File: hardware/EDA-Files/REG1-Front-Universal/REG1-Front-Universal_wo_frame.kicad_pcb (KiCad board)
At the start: 2 copper layers, 15.3 x 42.6 mm, 18 parts, among them J1 Frontpanel, SW1 Prog, SW2 Btn1, SW3 Res, SW4 BL

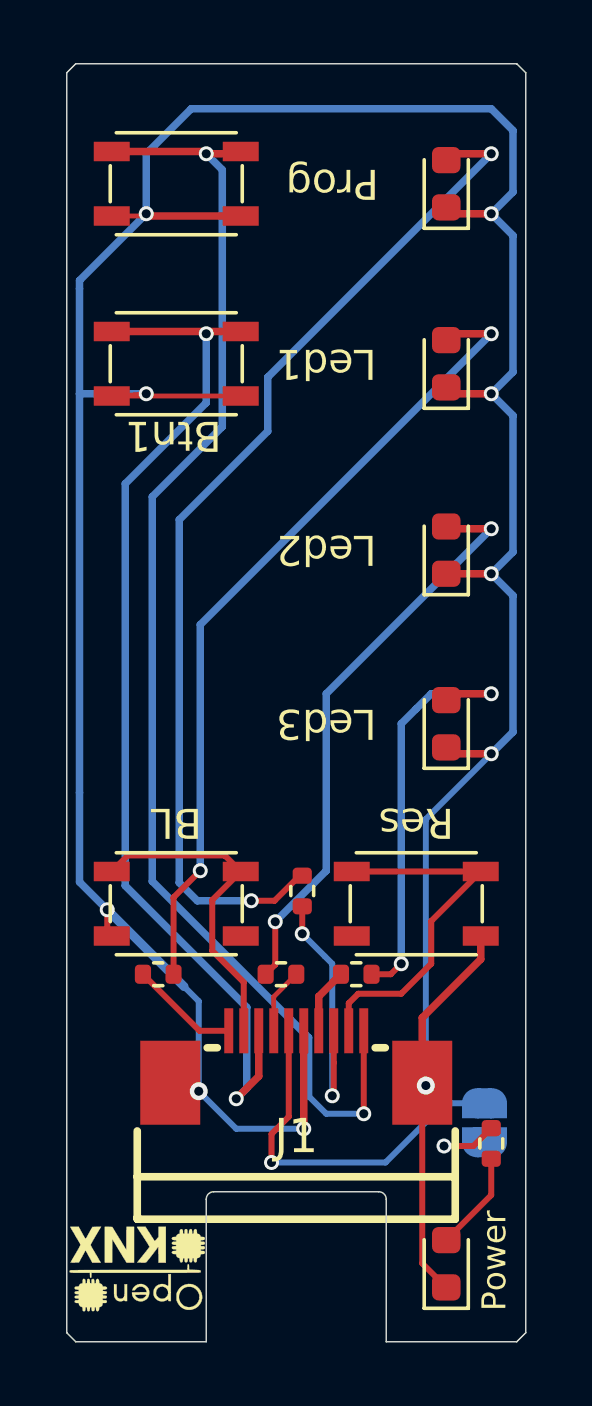
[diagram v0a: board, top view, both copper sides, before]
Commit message: new V01.00 (some 0.1 bigger)
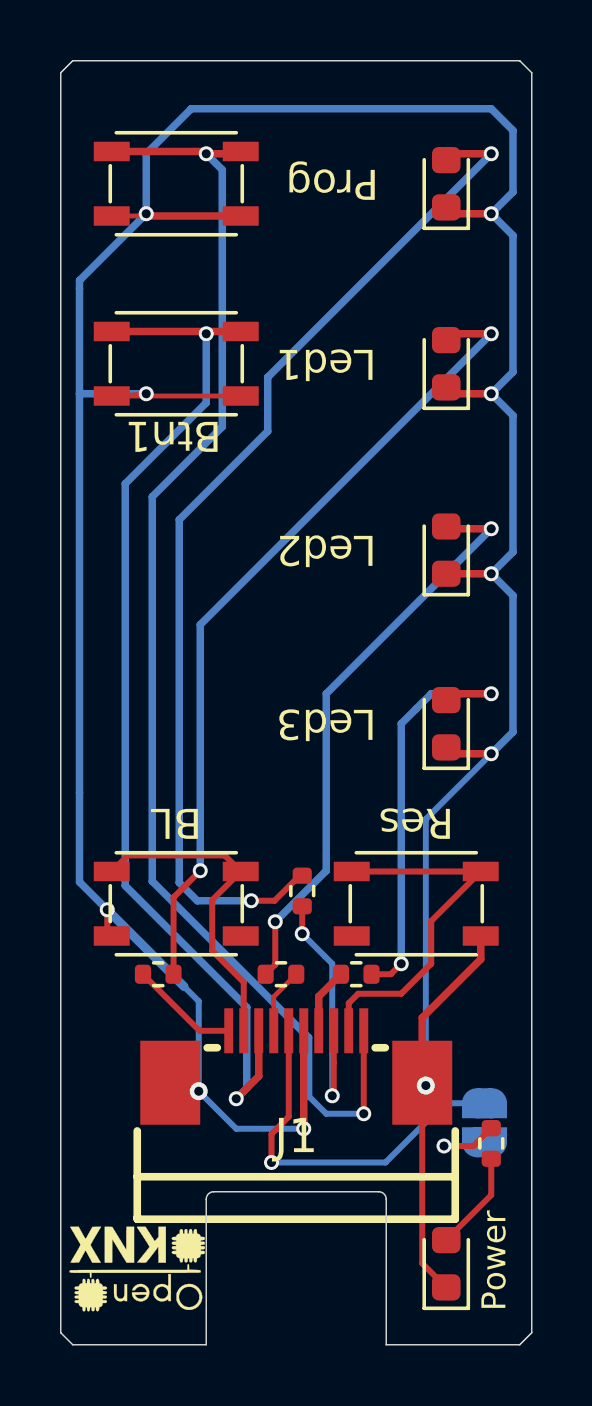
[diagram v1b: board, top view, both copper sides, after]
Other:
- board size 15.3 x 42.6 mm -> 15.7 x 42.8 mm
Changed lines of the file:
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@@
       (drillshape 0)
       (scaleselection 1)
-      (outputdirectory "REG1-Front-Universal_gerbers_V01.00/")
+      (outputdirectory "dxf/")
     )
   )
@@
   (gr_line (start 58.325 83) (end 60.225 83)
     (stroke (width 0.1) (type default)) (layer "Eco1.User"))
-  (gr_line (start 46.35 85.3) (end 46.35 43.3)
+  (gr_line (start 46.15 85.3) (end 46.15 43.3)
     (stroke (width 0.05) (type solid)) (layer "Edge.Cuts"))
-  (gr_line (start 61.35 43) (end 46.65 43)
+  (gr_line (start 61.45 85.7) (end 57 85.7)
+    (stroke (width 0.05) (type solid)) (layer "Edge.Cuts"))
+  (gr_line (start 51 85.7) (end 46.55 85.7)
+    (stroke (width 0.05) (type solid)) (layer "Edge.Cuts"))
+  (gr_line (start 61.45 42.9) (end 46.55 42.9)
     (stroke (width 0.05) (type default)) (layer "Edge.Cuts"))
-  (gr_line (start 46.65 43) (end 46.35 43.3)
+  (gr_line (start 46.55 42.9) (end 46.15 43.3)
     (stroke (width 0.05) (type solid)) (layer "Edge.Cuts"))
-  (gr_line (start 61.65 85.3) (end 61.35 85.6)
+  (gr_line (start 61.85 85.3) (end 61.45 85.7)
     (stroke (width 0.05) (type solid)) (layer "Edge.Cuts"))
-  (gr_line (start 46.65 85.6) (end 46.35 85.3)
+  (gr_line (start 46.55 85.7) (end 46.15 85.3)
     (stroke (width 0.05) (type default)) (layer "Edge.Cuts"))
   (gr_line (start 51.25 80.6) (end 56.75 80.6)
     (stroke (width 0.05) (type default)) (layer "Edge.Cuts"))
-  (gr_line (start 61.65 43.3) (end 61.65 85.3)
+  (gr_line (start 61.85 43.3) (end 61.85 85.3)
     (stroke (width 0.05) (type solid)) (layer "Edge.Cuts"))
-  (gr_line (start 51 85.6) (end 51 80.85)
-    (stroke (width 0.05) (type default)) (layer "Edge.Cuts"))
-  (gr_line (start 61.35 85.6) (end 57 85.6)
+  (gr_line (start 51 85.7) (end 51 80.85)
     (stroke (width 0.05) (type default)) (layer "Edge.Cuts"))
   (gr_arc (start 56.75 80.6) (mid 56.926777 80.673223) (end 57 80.85)
     (stroke (width 0.05) (type default)) (layer "Edge.Cuts"))
-  (gr_line (start 57 80.85) (end 57 85.6)
-    (stroke (width 0.05) (type default)) (layer "Edge.Cuts"))
-  (gr_line (start 51 85.6) (end 46.65 85.6)
+  (gr_line (start 57 80.85) (end 57 85.7)
     (stroke (width 0.05) (type default)) (layer "Edge.Cuts"))
-  (gr_line (start 61.35 43) (end 61.65 43.3)
+  (gr_line (start 61.45 42.9) (end 61.85 43.3)
     (stroke (width 0.05) (type default)) (layer "Edge.Cuts"))
   (gr_arc (start 51 80.85) (mid 51.073223 80.673223) (end 51.25 80.6)
